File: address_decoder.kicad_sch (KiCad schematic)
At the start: 9 parts, among them J1 Conn_02x04_Counter_Clockwise, U2 74LS138, U3 74LS245, U4 74LS08, U5 74LS02, U6 74LS00, U7 PAL16L8, U8 74LS08

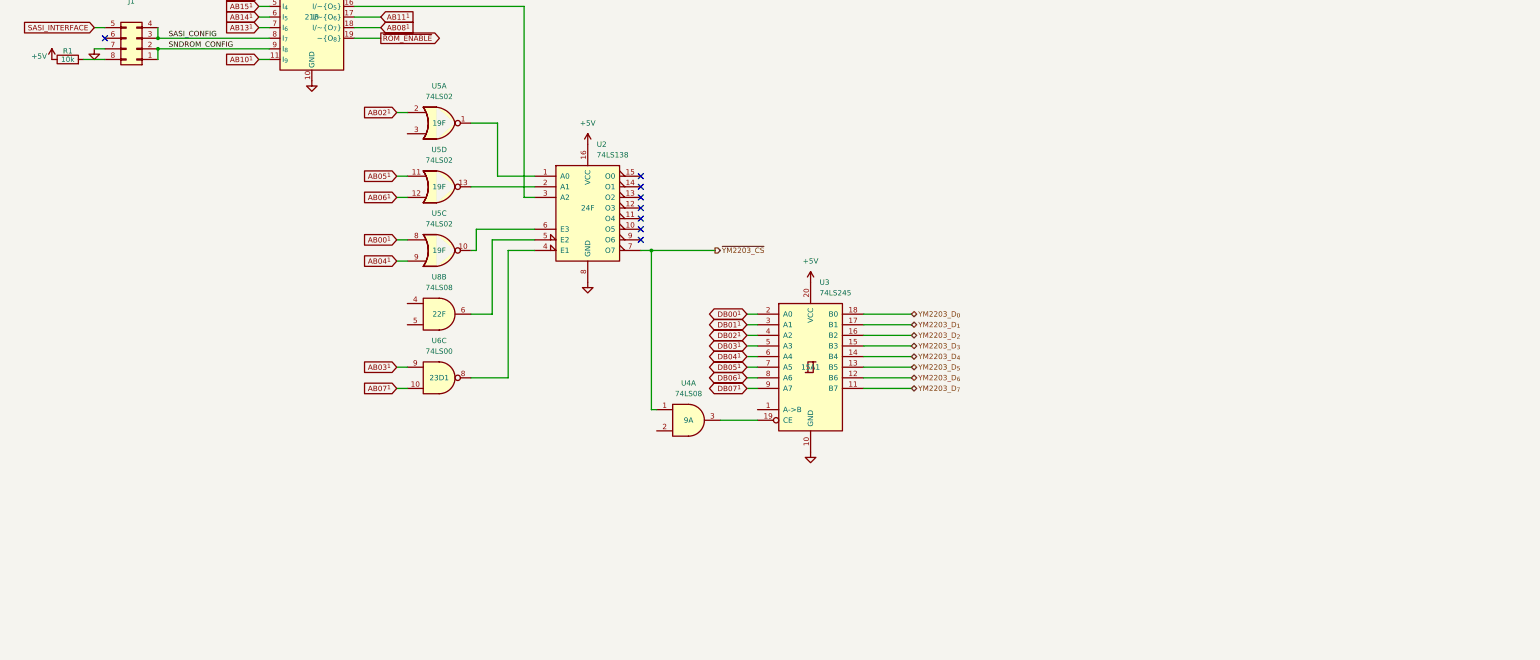
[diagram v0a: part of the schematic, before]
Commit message: Update circuit
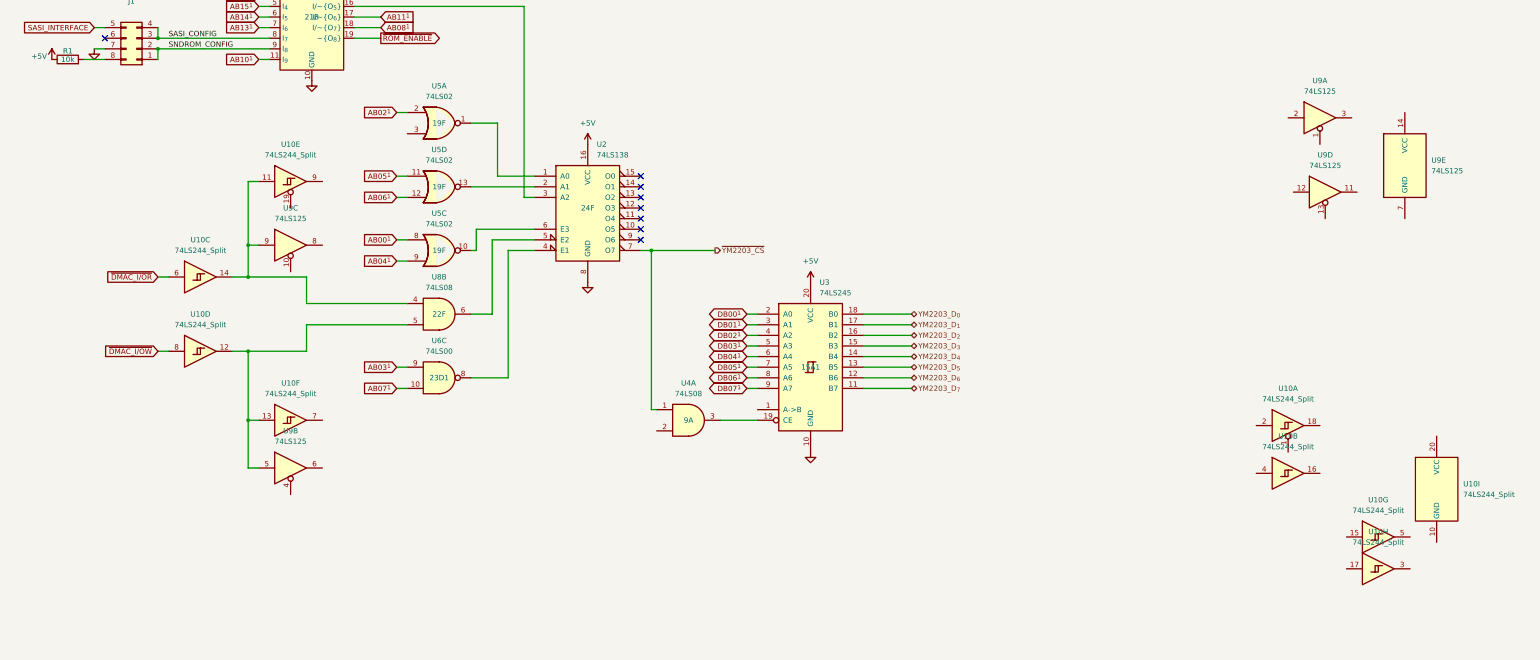
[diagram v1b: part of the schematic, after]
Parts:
- added U10: 74LS244_Split, symbol 74xx:74LS244_Split
- added U9: 74LS125, symbol 74xx:74LS125
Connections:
- net at U8.4: now also U10.11, U10.14, U9.9
- net at U8.5: now also U10.12, U10.13, U9.5
- new net ~{DMAC_I/OR}: U10.6
- new net ~{DMAC_I/OW}: U10.8
